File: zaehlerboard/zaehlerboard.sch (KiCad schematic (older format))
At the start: 10 parts, among them Q1 Q_Photo_NPN, U1 ESP1, U2 MCP1700-3.3, U3 LM293

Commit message: pin associations
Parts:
- C1: footprint Capacitor_THT:CP_Radial_D8.0mm_P5.00mm -> Capacitor_THT:C_Disc_D5.0mm_W2.5mm_P5.00mm
- R1, R2, R3: footprint (none) -> Resistor_THT:R_Axial_DIN0204_L3.6mm_D1.6mm_P7.62mm_Horizontal
- RV1: footprint (none) -> Potentiometer_THT:Potentiometer_ACP_CA9-V10_Vertical
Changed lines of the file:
@@
 F 0 "R2" H 5820 3396 50  0000 L CNN
 F 1 "22k" H 5820 3305 50  0000 L CNN
-F 2 "" V 5680 3350 50  0001 C CNN
+F 2 "Resistor_THT:R_Axial_DIN0204_L3.6mm_D1.6mm_P7.62mm_Horizontal" V 5680 3350 50  0001 C CNN
 F 3 "~" H 5750 3350 50  0001 C CNN
 	1    5750 3350
@@
 F 0 "R1" H 4630 3304 50  0000 R CNN
 F 1 "43" H 4630 3395 50  0000 R CNN
-F 2 "" V 4630 3350 50  0001 C CNN
+F 2 "Resistor_THT:R_Axial_DIN0204_L3.6mm_D1.6mm_P7.62mm_Horizontal" V 4630 3350 50  0001 C CNN
 F 3 "~" H 4700 3350 50  0001 C CNN
 	1    4700 3350
@@
 F 0 "RV1" V 6793 2550 50  0000 C CNN
 F 1 "10k" V 6884 2550 50  0000 C CNN
-F 2 "" H 7000 2550 50  0001 C CNN
+F 2 "Potentiometer_THT:Potentiometer_ACP_CA9-V10_Vertical" H 7000 2550 50  0001 C CNN
 F 3 "~" H 7000 2550 50  0001 C CNN
 	1    7000 2550
@@
 F 0 "C1" H 8465 3296 50  0000 L CNN
 F 1 "100nF" H 8465 3205 50  0000 L CNN
-F 2 "Capacitor_THT:CP_Radial_D8.0mm_P5.00mm" H 8388 3100 50  0001 C CNN
+F 2 "Capacitor_THT:C_Disc_D5.0mm_W2.5mm_P5.00mm" H 8388 3100 50  0001 C CNN
 F 3 "~" H 8350 3250 50  0001 C CNN
 	1    8350 3250
@@
 F 0 "R3" V 9843 1150 50  0000 C CNN
 F 1 "3k3" V 9934 1150 50  0000 C CNN
-F 2 "" V 9980 1150 50  0001 C CNN
+F 2 "Resistor_THT:R_Axial_DIN0204_L3.6mm_D1.6mm_P7.62mm_Horizontal" V 9980 1150 50  0001 C CNN
 F 3 "~" H 10050 1150 50  0001 C CNN
 	1    10050 1150

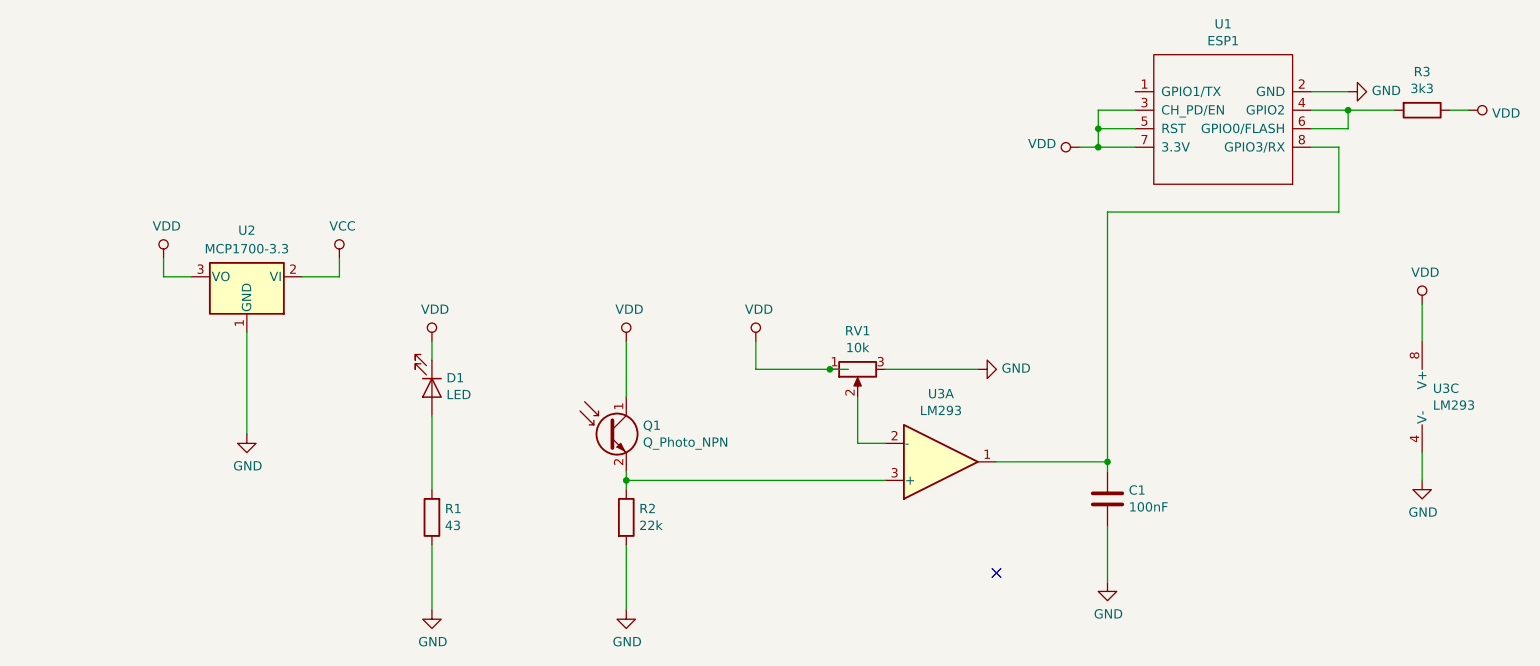
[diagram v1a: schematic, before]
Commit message: update circuit
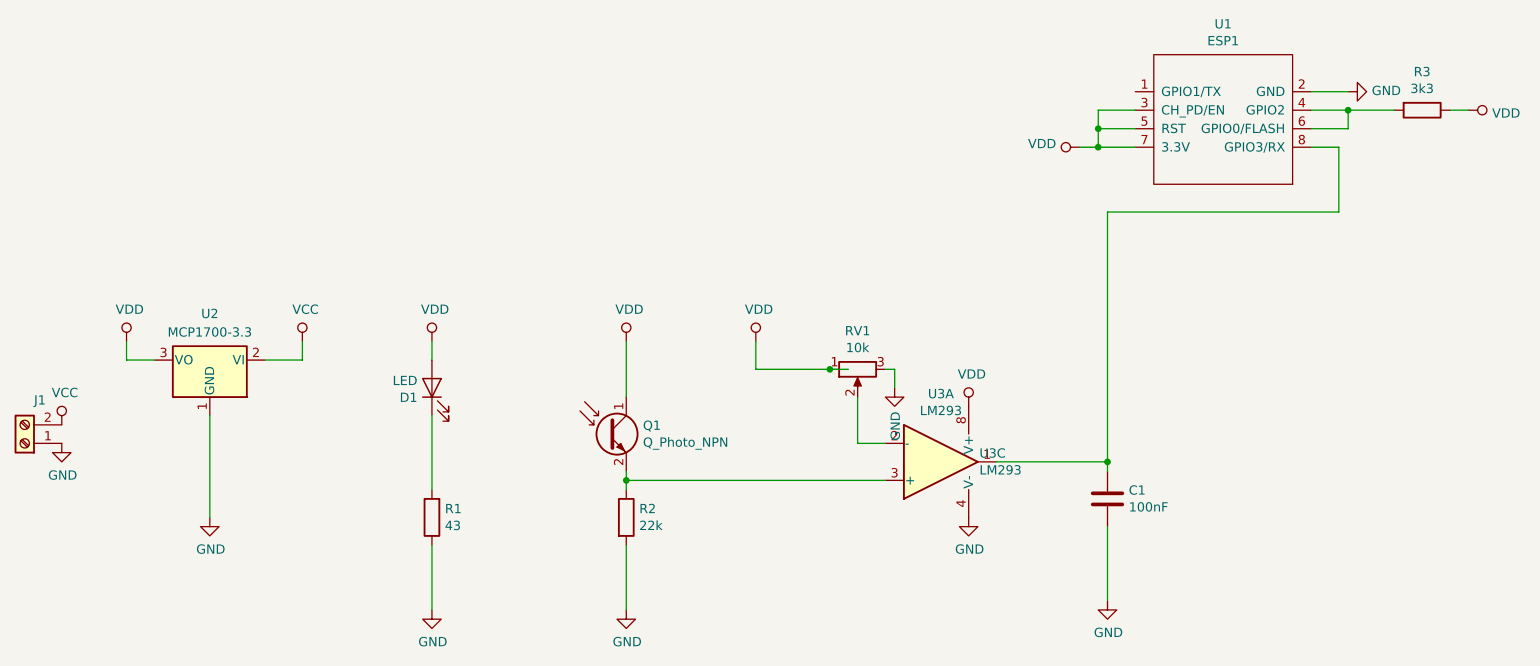
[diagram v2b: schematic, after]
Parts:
- added J1: Screw_Terminal_01x02, TerminalBlock:TerminalBlock_Altech_AK300-2_P5.00mm, symbol Connector:Screw_Terminal_01x02
- RV1: footprint Potentiometer_THT:Potentiometer_ACP_CA9-V10_Vertical -> Potentiometer_THT:Potentiometer_ACP_CA9-H5_Horizontal
- U3: footprint Package_DIP:DIP-8_W10.16mm -> Package_DIP:DIP-8_W7.62mm_Socket
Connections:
- net GND: now also J1.1 (Pin_1)
- net VCC: now also J1.2 (Pin_2)
- net VDD: now also D1.2 (A); no longer D1.1 (K)
- net at R1.2: now also D1.1 (K); no longer D1.2 (A)
- no-connect marks 1 -> 0
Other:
- moved on the sheet: D1, U2, U3C
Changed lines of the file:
@@
 F 3 "~" H 4700 2650 50  0001 C CNN
 	1    4700 2650
-	0    1    1    0
+	0    -1   -1   0
 $EndComp
 $Comp
@@
 F 0 "U3" H 7450 2683 50  0000 C CNN
 F 1 "LM293" H 7450 2774 50  0000 C CNN
-F 2 "Package_DIP:DIP-8_W10.16mm" H 7400 3150 50  0001 C CNN
+F 2 "Package_DIP:DIP-8_W7.62mm_Socket" H 7400 3150 50  0001 C CNN
 F 3 "http://www.ti.com/lit/ds/symlink/tl081.pdf" H 7500 3250 50  0001 C CNN
 	1    7450 3050
@@
 	1    0    0    -1
 $EndComp
-$Comp
-L power:GND #PWR0105
-U 1 1 5D3768AA
-P 7650 2550
-F 0 "#PWR0105" H 7650 2300 50  0001 C CNN
-F 1 "GND" V 7655 2422 50  0000 R CNN
-F 2 "" H 7650 2550 50  0001 C CNN
-F 3 "" H 7650 2550 50  0001 C CNN
-	1    7650 2550
-	0    -1   -1   0
-$EndComp
 Wire Wire Line
 	6450 2550 6450 2400
@@
 L Regulator_Linear:MCP1700-3302E_TO92 U2
 U 1 1 5D3977D9
-P 3700 2050
-F 0 "U2" H 3700 1800 50  0000 C CNN
-F 1 "MCP1700-3.3" H 3700 1900 50  0000 C CNN
-F 2 "Package_TO_SOT_THT:TO-92" H 3700 2300 50  0001 C CIN
-F 3 "http://www.ti.com/lit/ds/symlink/lm1085.pdf" H 3700 2050 50  0001 C CNN
-	1    3700 2050
+P 3500 2500
+F 0 "U2" H 3500 2250 50  0000 C CNN
+F 1 "MCP1700-3.3" H 3500 2350 50  0000 C CNN
+F 2 "Package_TO_SOT_THT:TO-92" H 3500 2750 50  0001 C CIN
+F 3 "http://www.ti.com/lit/ds/symlink/lm1085.pdf" H 3500 2500 50  0001 C CNN
+	1    3500 2500
 	-1   0    0    1
 $EndComp
@@
 L power:GND #PWR02
 U 1 1 5D39ABD9
-P 3700 2900
-F 0 "#PWR02" H 3700 2650 50  0001 C CNN
-F 1 "GND" H 3705 2727 50  0000 C CNN
-F 2 "" H 3700 2900 50  0001 C CNN
-F 3 "" H 3700 2900 50  0001 C CNN
-	1    3700 2900
+P 3500 3350
+F 0 "#PWR02" H 3500 3100 50  0001 C CNN
+F 1 "GND" H 3505 3177 50  0000 C CNN
+F 2 "" H 3500 3350 50  0001 C CNN
+F 3 "" H 3500 3350 50  0001 C CNN
+	1    3500 3350
 	1    0    0    -1
 $EndComp
@@
 L power:VDD #PWR03
 U 1 1 5D39B7A3
-P 3250 1950
-F 0 "#PWR03" H 3250 1800 50  0001 C CNN
-F 1 "VDD" H 3267 2123 50  0000 C CNN
-F 2 "" H 3250 1950 50  0001 C CNN
-F 3 "" H 3250 1950 50  0001 C CNN
-	1    3250 1950
+P 3050 2400
+F 0 "#PWR03" H 3050 2250 50  0001 C CNN
+F 1 "VDD" H 3067 2573 50  0000 C CNN
+F 2 "" H 3050 2400 50  0001 C CNN
+F 3 "" H 3050 2400 50  0001 C CNN
+	1    3050 2400
 	1    0    0    -1
 $EndComp
@@
 L power:VCC #PWR01
 U 1 1 5D39C377
-P 4200 1950
-F 0 "#PWR01" H 4200 1800 50  0001 C CNN
-F 1 "VCC" H 4217 2123 50  0000 C CNN
-F 2 "" H 4200 1950 50  0001 C CNN
-F 3 "" H 4200 1950 50  0001 C CNN
-	1    4200 1950
+P 4000 2400
+F 0 "#PWR01" H 4000 2250 50  0001 C CNN
+F 1 "VCC" H 4017 2573 50  0000 C CNN
+F 2 "" H 4000 2400 50  0001 C CNN
+F 3 "" H 4000 2400 50  0001 C CNN
+	1    4000 2400
 	1    0    0    -1
 $EndComp
@@
 F 0 "RV1" V 6793 2550 50  0000 C CNN
 F 1 "10k" V 6884 2550 50  0000 C CNN
-F 2 "Potentiometer_THT:Potentiometer_ACP_CA9-V10_Vertical" H 7000 2550 50  0001 C CNN
+F 2 "Potentiometer_THT:Potentiometer_ACP_CA9-H5_Horizontal" H 7000 2550 50  0001 C CNN
 F 3 "~" H 7000 2550 50  0001 C CNN
 	1    7000 2550
@@
 Wire Wire Line
 	7000 2700 7000 2950
-NoConn ~ 7750 3650
-Wire Wire Line
-	7150 2550 7650 2550
+Wire Wire Line
+	7150 2550 7200 2550
 $Comp
 L Amplifier_Operational:LM2904 U3
 U 3 1 5D890418
-P 10150 2700
-F 0 "U3" H 10108 2746 50  0000 L CNN
-F 1 "LM293" H 10108 2655 50  0000 L CNN
-F 2 "Package_DIP:DIP-8_W10.16mm" H 10150 2700 50  0001 C CNN
-F 3 "http://www.ti.com/lit/ds/symlink/tl081.pdf" H 10150 2700 50  0001 C CNN
-	3    10150 2700
+P 7700 3050
+F 0 "U3" H 7658 3096 50  0000 L CNN
+F 1 "LM293" H 7658 3005 50  0000 L CNN
+F 2 "Package_DIP:DIP-8_W7.62mm_Socket" H 7700 3050 50  0001 C CNN
+F 3 "http://www.ti.com/lit/ds/symlink/tl081.pdf" H 7700 3050 50  0001 C CNN
+	3    7700 3050
 	1    0    0    -1
 $EndComp
@@
 L power:VDD #PWR04
 U 1 1 5D893A2A
-P 10050 2200
-F 0 "#PWR04" H 10050 2050 50  0001 C CNN
-F 1 "VDD" H 10067 2373 50  0000 C CNN
-F 2 "" H 10050 2200 50  0001 C CNN
-F 3 "" H 10050 2200 50  0001 C CNN
-	1    10050 2200
+P 7600 2750
+F 0 "#PWR04" H 7600 2600 50  0001 C CNN
+F 1 "VDD" H 7617 2923 50  0000 C CNN
+F 2 "" H 7600 2750 50  0001 C CNN
+F 3 "" H 7600 2750 50  0001 C CNN
+	1    7600 2750
 	1    0    0    -1
 $EndComp
@@
 L power:GND #PWR05
 U 1 1 5D894387
-P 10050 3150
-F 0 "#PWR05" H 10050 2900 50  0001 C CNN
-F 1 "GND" H 10055 2977 50  0000 C CNN
-F 2 "" H 10050 3150 50  0001 C CNN
-F 3 "" H 10050 3150 50  0001 C CNN
-	1    10050 3150
-	1    0    0    -1
-$EndComp
-Wire Wire Line
-	10050 2400 10050 2200
-Wire Wire Line
-	10050 3150 10050 3000
+P 7600 3350
+F 0 "#PWR05" H 7600 3100 50  0001 C CNN
+F 1 "GND" H 7605 3177 50  0000 C CNN
+F 2 "" H 7600 3350 50  0001 C CNN
+F 3 "" H 7600 3350 50  0001 C CNN
+	1    7600 3350
+	1    0    0    -1
+$EndComp
 $Comp
 L Device:C C1
@@
 F 3 "~" H 8350 3250 50  0001 C CNN
 	1    8350 3250
-	1    0    0    -1
-$EndComp
-$Comp
-L power:GND #PWR07
-U 1 1 5D89E950
-P 8350 3700
-F 0 "#PWR07" H 8350 3450 50  0001 C CNN
-F 1 "GND" H 8355 3527 50  0000 C CNN
-F 2 "" H 8350 3700 50  0001 C CNN
-F 3 "" H 8350 3700 50  0001 C CNN
-	1    8350 3700
 	1    0    0    -1
 $EndComp
@@
 	8350 3050 8350 3100
 Wire Wire Line
-	8350 3400 8350 3700
-Wire Wire Line
 	8350 3050 8350 1700
 Wire Wire Line
@@
 	9450 1050 9650 1050
 Wire Wire Line
-	3250 1950 3250 2050
-Wire Wire Line
-	3250 2050 3400 2050
-Wire Wire Line
-	4200 1950 4200 2050
-Wire Wire Line
-	4200 2050 4000 2050
-Wire Wire Line
-	3700 2350 3700 2900
+	3050 2400 3050 2500
+Wire Wire Line
+	3050 2500 3200 2500
+Wire Wire Line
+	4000 2400 4000 2500
+Wire Wire Line
+	4000 2500 3800 2500
+Wire Wire Line
+	3500 2800 3500 3350
+$Comp
+L Connector:Screw_Terminal_01x02 J1
+U 1 1 5D8B0312
+P 2500 2950
+F 0 "J1" H 2418 2717 50  0000 C CNN
+F 1 "Screw_Terminal_01x02" H 2418 2716 50  0001 C CNN
+F 2 "TerminalBlock:TerminalBlock_Altech_AK300-2_P5.00mm" H 2500 2950 50  0001 C CNN
+F 3 "~" H 2500 2950 50  0001 C CNN
+	1    2500 2950
+	-1   0    0    1
+$EndComp
+$Comp
+L power:GND #PWR0105
+U 1 1 5D3768AA
+P 7200 2650
+F 0 "#PWR0105" H 7200 2400 50  0001 C CNN
+F 1 "GND" V 7205 2522 50  0000 R CNN
+F 2 "" H 7200 2650 50  0001 C CNN
+F 3 "" H 7200 2650 50  0001 C CNN
+	1    7200 2650
+	1    0    0    -1
+$EndComp
+Wire Wire Line
+	7200 2650 7200 2550
+$Comp
+L power:VCC #PWR0106
+U 1 1 5D8F6DB0
+P 2700 2850
+F 0 "#PWR0106" H 2700 2700 50  0001 C CNN
+F 1 "VCC" H 2717 3023 50  0000 C CNN
+F 2 "" H 2700 2850 50  0001 C CNN
+F 3 "" H 2700 2850 50  0001 C CNN
+	1    2700 2850
+	1    0    0    -1
+$EndComp
+$Comp
+L power:GND #PWR0108
+U 1 1 5D8F783F
+P 2700 2950
+F 0 "#PWR0108" H 2700 2700 50  0001 C CNN
+F 1 "GND" H 2705 2777 50  0000 C CNN
+F 2 "" H 2700 2950 50  0001 C CNN
+F 3 "" H 2700 2950 50  0001 C CNN
+	1    2700 2950
+	1    0    0    -1
+$EndComp
+$Comp
+L power:GND #PWR07
+U 1 1 5D89E950
+P 8350 3800
+F 0 "#PWR07" H 8350 3550 50  0001 C CNN
+F 1 "GND" H 8355 3627 50  0000 C CNN
+F 2 "" H 8350 3800 50  0001 C CNN
+F 3 "" H 8350 3800 50  0001 C CNN
+	1    8350 3800
+	1    0    0    -1
+$EndComp
+Wire Wire Line
+	8350 3400 8350 3800
 $EndSCHEMATC
